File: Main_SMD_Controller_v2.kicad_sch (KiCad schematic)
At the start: 55 parts, among them J1 Vsens, J10 Switch_Control, J2 VsensJMP, J3 Vin+, J4 Drain, J5 AnalogIO, J6 Conn_01x02, J7 Gate, J8 Source, J9 Vin_-, P1 Eoshi-chan_Silk, P2 Eoshi-chan_Silk, P3 Serial_QR, Q1 2N7002K, U1 ADA4075-2, U2 ADA4522-1, U3 TC74HC4066AP, U4 ADA4510-2ARZ, U5 74AHC1G04

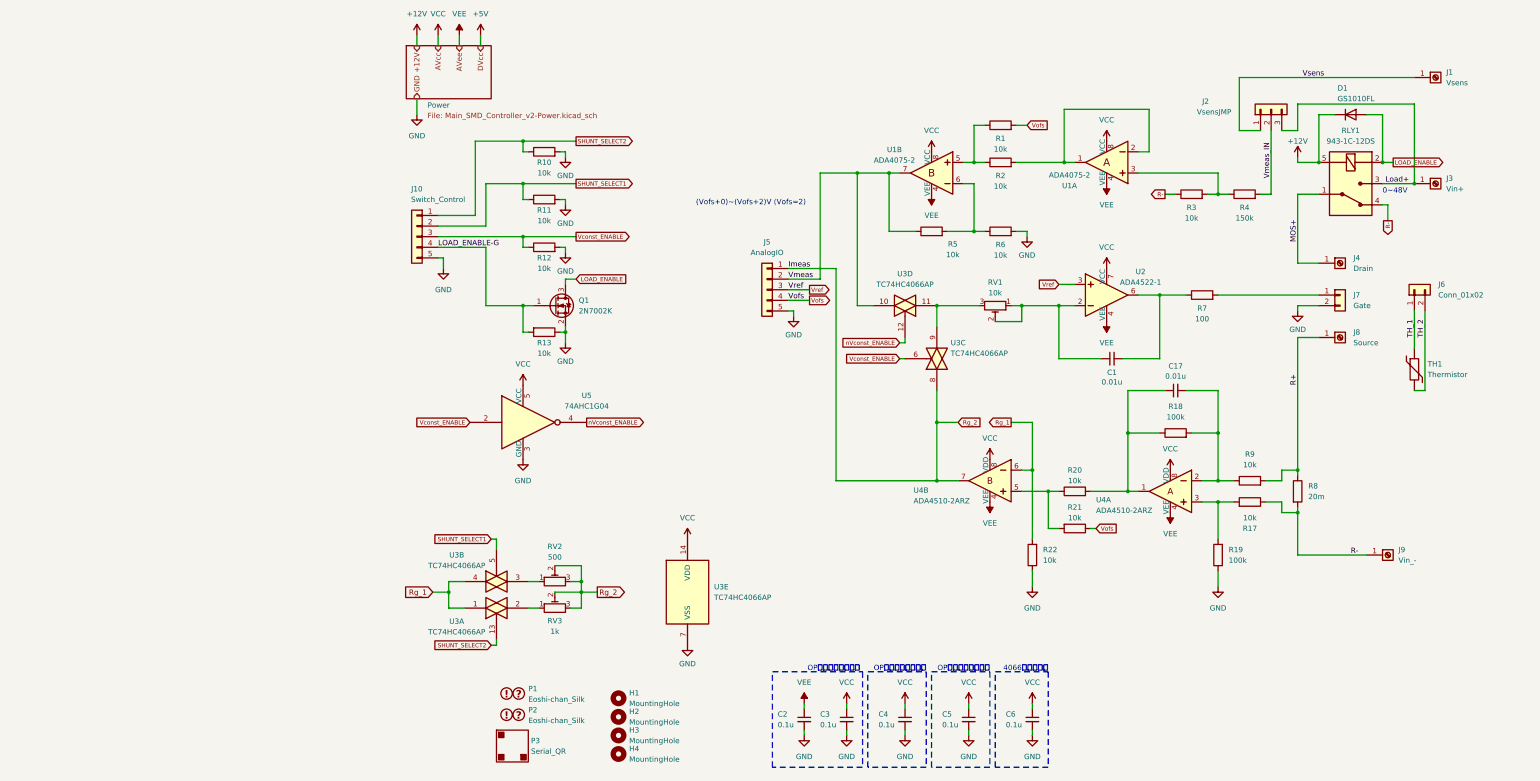
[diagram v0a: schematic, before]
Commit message: up
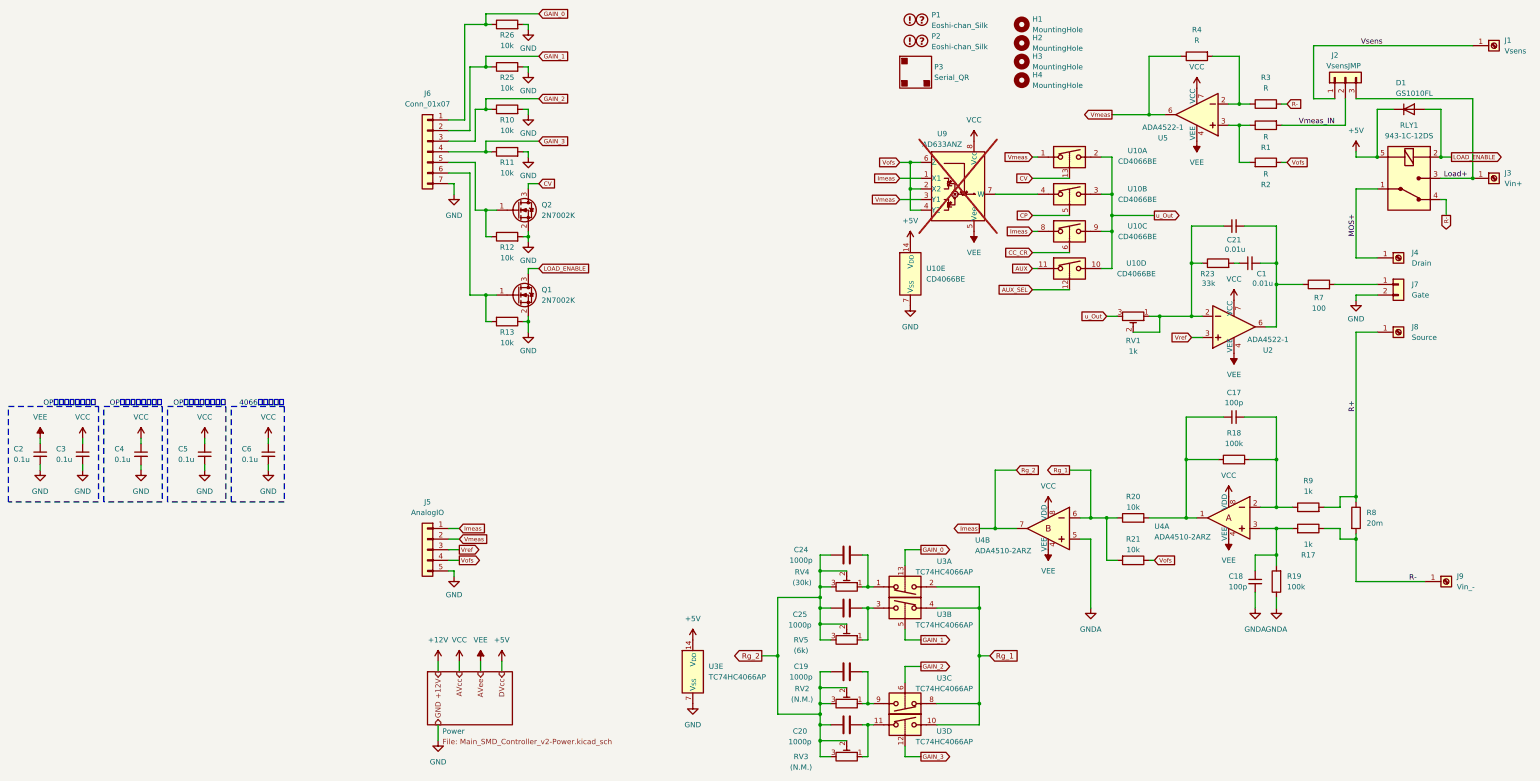
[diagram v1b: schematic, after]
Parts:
- removed J10: Switch_Control, Connector_JST:JST_XH_B5B-XH-A_1x05_P2.50mm_Vertical, symbol Connector_Generic:Conn_01x05
- removed J6: Conn_01x02, Connector_JST:JST_XH_B2B-XH-A_1x02_P2.50mm_Vertical, symbol Connector_Generic:Conn_01x02
- removed R22: 10k, symbol Device:R
- removed R5, R6: 10k, Resistor_SMD:R_0603_1608Metric, symbol Device:R
- removed TH1: Thermistor, Capacitor_THT:C_Disc_D3.0mm_W1.6mm_P2.50mm, symbol Device:Thermistor
- removed U1: ADA4075-2, Package_SO:SOIC-8_3.9x4.9mm_P1.27mm, symbol Amplifier_Operational:ADA4075-2
- removed U3: TC74HC4066AP, Package_DIP:DIP-14_W7.62mm_Socket, symbol 4xxx:4066
- removed U5: 74AHC1G04, Package_TO_SOT_SMD:SOT-23-5, symbol 74xGxx:74AHC1G04
- added C18: 100p, Capacitor_SMD:C_0603_1608Metric, symbol Device:C_Small
- added C19, C20, C24, C25: 1000p, symbol Device:C
- added C21: 0.01u, Capacitor_SMD:C_0402_1005Metric, symbol Device:C_Small
- added J6: Conn_01x07, Connector_JST:JST_XH_B7B-XH-A_1x07_P2.50mm_Vertical, symbol Connector_Generic:Conn_01x07
- added Q2: 2N7002K, Package_TO_SOT_SMD:SOT-23, symbol Transistor_FET:2N7002K
- added R23: 33k, symbol Device:R
- added R25, R26: 10k, Resistor_SMD:R_0603_1608Metric, symbol Device:R
- added RV4: (30k), Potentiometer_THT:Potentiometer_Bourns_3296W_Vertical, symbol Device:R_Potentiometer_Trim
- added RV5: (6k), Potentiometer_THT:Potentiometer_Bourns_3296W_Vertical, symbol Device:R_Potentiometer_Trim
- added U10: CD4066BE, Package_DIP:DIP-14_W7.62mm, symbol Analog_Switch:CD4066BE
- added U3: TC74HC4066AP, Package_DIP:DIP-14_W7.62mm, symbol Analog_Switch:CD4066BE
- added U5: ADA4522-1, Package_SO:SOIC-8_3.9x4.9mm_P1.27mm, symbol Amplifier_Operational:ADA4522-1
- added U9: AD633ANZ, Package_DIP:DIP-8_W7.62mm, symbol AM_Opamp:AD633ANZ
- C17: value 0.01u -> 100p
- R1, R2: value 10k -> R; footprint Resistor_SMD:R_0603_1608Metric -> (none)
- R17, R9, RV1: value 10k -> 1k
- R3: value 10k -> R; footprint Resistor_THT:R_Axial_DIN0207_L6.3mm_D2.5mm_P10.16mm_Horizontal -> (none)
- R4: value 150k -> R; footprint Resistor_THT:R_Axial_DIN0207_L6.3mm_D2.5mm_P10.16mm_Horizontal -> (none)
- RV2: value 500 -> (N.M.)
- RV3: value 1k -> (N.M.)
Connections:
- net +12V: no longer D1.1 (K), RLY1.5 (COIL)
- net +5V: now also D1.1 (K), RLY1.5 (COIL), U10.14 (V_{DD}), U3.14 (V_{DD})
- net GND: now also J6.7 (Pin_7), Q2.2 (S), R25.2, R26.2, U10.7 (V_{SS}), U3.7 (V_{SS}); no longer R19.1
- net R-: now also R3.2; no longer R3.1
- net Rg_1: now also R20.1, R21.2, U3.10, U3.2, U3.4, U3.8
- net VCC: now also U5.7 (VCC), U9.8 (Vcc)
- net VEE: now also U5.4 (VEE), U9.5 (Vee)
- net Vmeas: now also R4.1, U10.1, U5.6, U9.3 (Y1)
- net Vmeas_IN: now also R1.2; no longer R4.2
- net Vofs: now also R2.1, U9.2 (X2), U9.4 (Y2), U9.6 (Z); no longer R1.2
- net at RV3.1: now also C20.1, U3.11
- net at R1.1: now also R2.2, U5.3; no longer R2.1
- net at R17.2, R19.2, U4.3: now also C18.1
- net u_Out: now reaches RV1.3
- net u_Out: now also U10.10, U10.2, U10.3, U10.9
- net at RV2.1: now also C19.1, U3.9
- net at C1.2, R7.1, U2.6: now also C21.2
- net at RV1.1, RV1.2, U2.2: now also C21.1, R23.1; no longer C1.1
- net LOAD_ENABLE-G: no longer names the net of Q1.1 (G), R13.2
- net LOAD_ENABLE-G: now also J6.6 (Pin_6)
- net Rg_2 renamed Imeas
- net Imeas: now also C19.2, C20.2, C24.2, C25.2, RV4.2, RV4.3, RV5.2, RV5.3, U10.8, U9.1 (X1)
- net SHUNT_SELECT1 renamed GAIN_3
- net GAIN_3: now also J6.4 (Pin_4), U3.12
- net SHUNT_SELECT2 renamed GAIN_2
- net GAIN_2: now also J6.3 (Pin_3), U3.6
- net Vconst_ENABLE: no longer names the net of R12.1
- net Vconst_ENABLE: now also J6.5 (Pin_5), Q2.1 (G)
- new net: C25.1, RV5.1, U3.3
- new net: U10.4, U9.7 (W)
- new net: C24.1, RV4.1, U3.1
- new net: R3.1, R4.2, U5.2
- new net: C1.1, R23.2
- new net AUX: U10.11
- new net AUX_SEL: U10.12
- new net CC_CR: U10.6
- new net CP: U10.5
- new net CV: Q2.3 (D), U10.13
- new net GAIN_0: J6.1 (Pin_1), R26.1, U3.13
- new net GAIN_1: J6.2 (Pin_2), R25.1, U3.5
- new net GNDA: C18.2, R19.1, U4.5
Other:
- note removed: "(Vofs+0)~(Vofs+2)V (Vofs=2)"
- note removed: "0~48V"
- moved on the sheet: C1, C17, C2, C3, C4, C5, C6, D1, H1, H2, H3, H4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

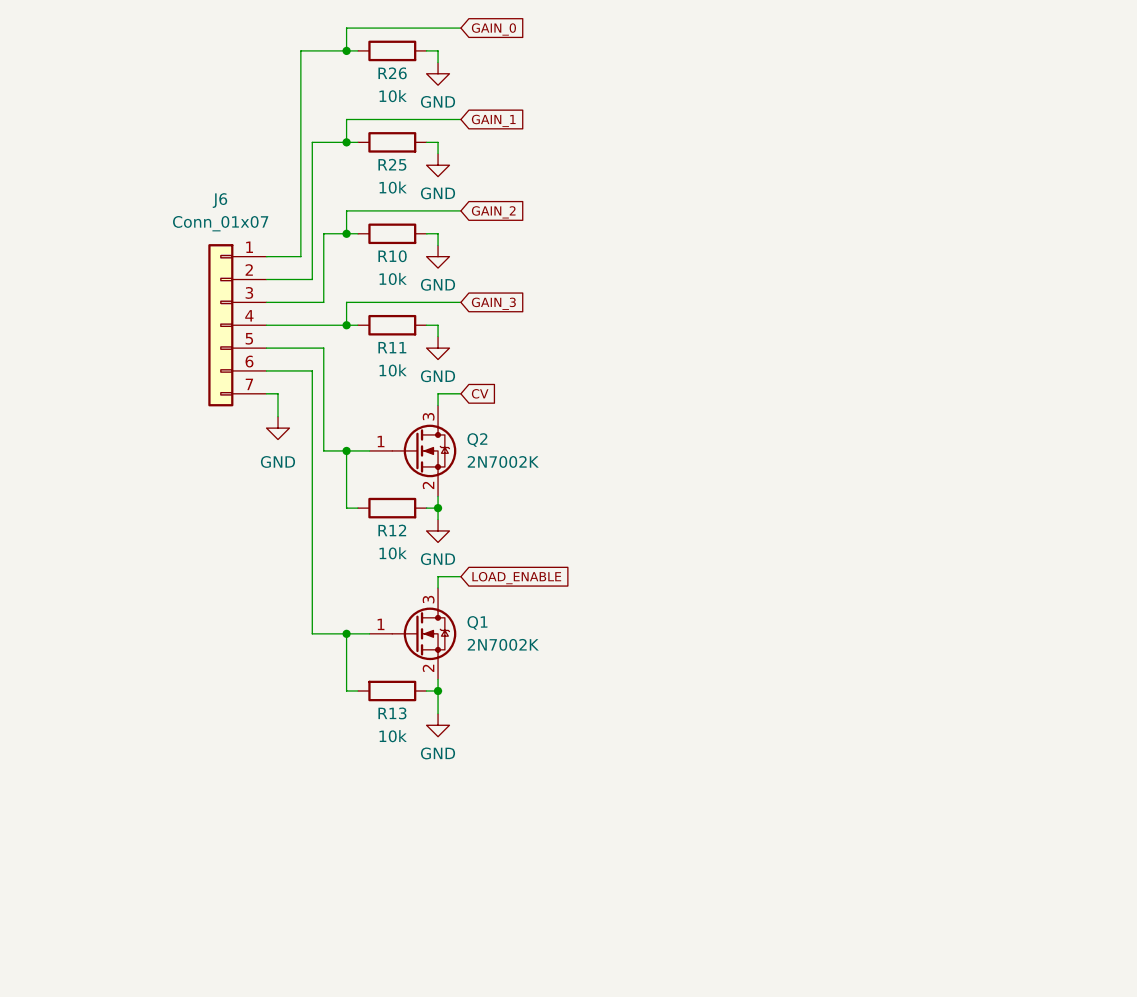
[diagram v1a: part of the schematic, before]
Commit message: unya
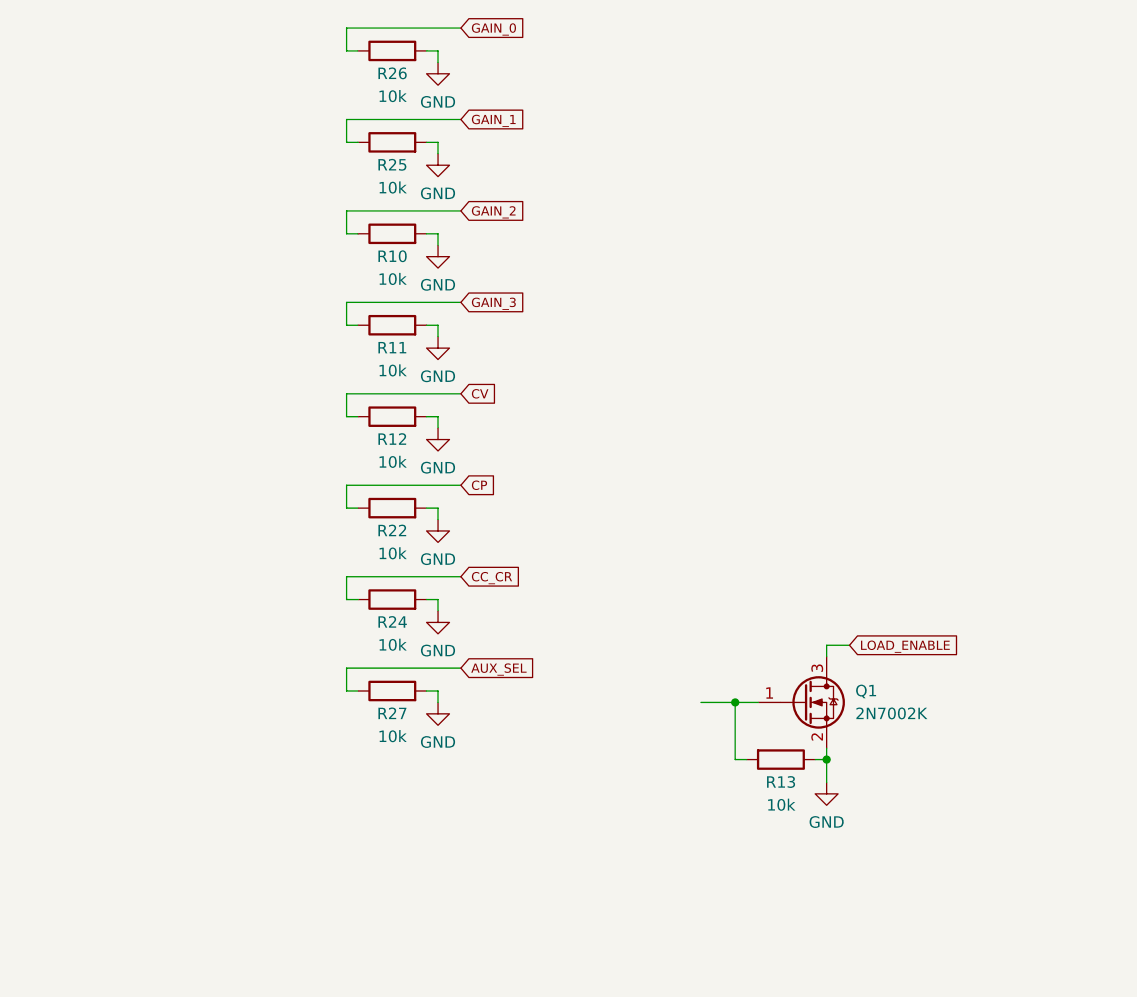
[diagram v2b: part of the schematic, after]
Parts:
- removed J6: Conn_01x07, Connector_JST:JST_XH_B7B-XH-A_1x07_P2.50mm_Vertical, symbol Connector_Generic:Conn_01x07
- removed Q2: 2N7002K, Package_TO_SOT_SMD:SOT-23, symbol Transistor_FET:2N7002K
- added R22, R24, R27: 10k, Resistor_SMD:R_0603_1608Metric, symbol Device:R
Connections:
- net AUX_SEL: now also R27.1
- net CC_CR: now also R24.1
- net CP: now also R22.1
- net CV: now also R12.1
- net GND: now also R22.2, R24.2, R27.2
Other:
- moved on the sheet: Q1, R12, R13
